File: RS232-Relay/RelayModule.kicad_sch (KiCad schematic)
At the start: 30 parts, among them J9 Relay 1-4, K1 G5V-1, K2 G5V-1, K3 G5V-1, K4 G5V-1, Q1 2N3904, Q2 2N3904, Q3 2N3904, Q4 2N3904, U6 LTV-847S

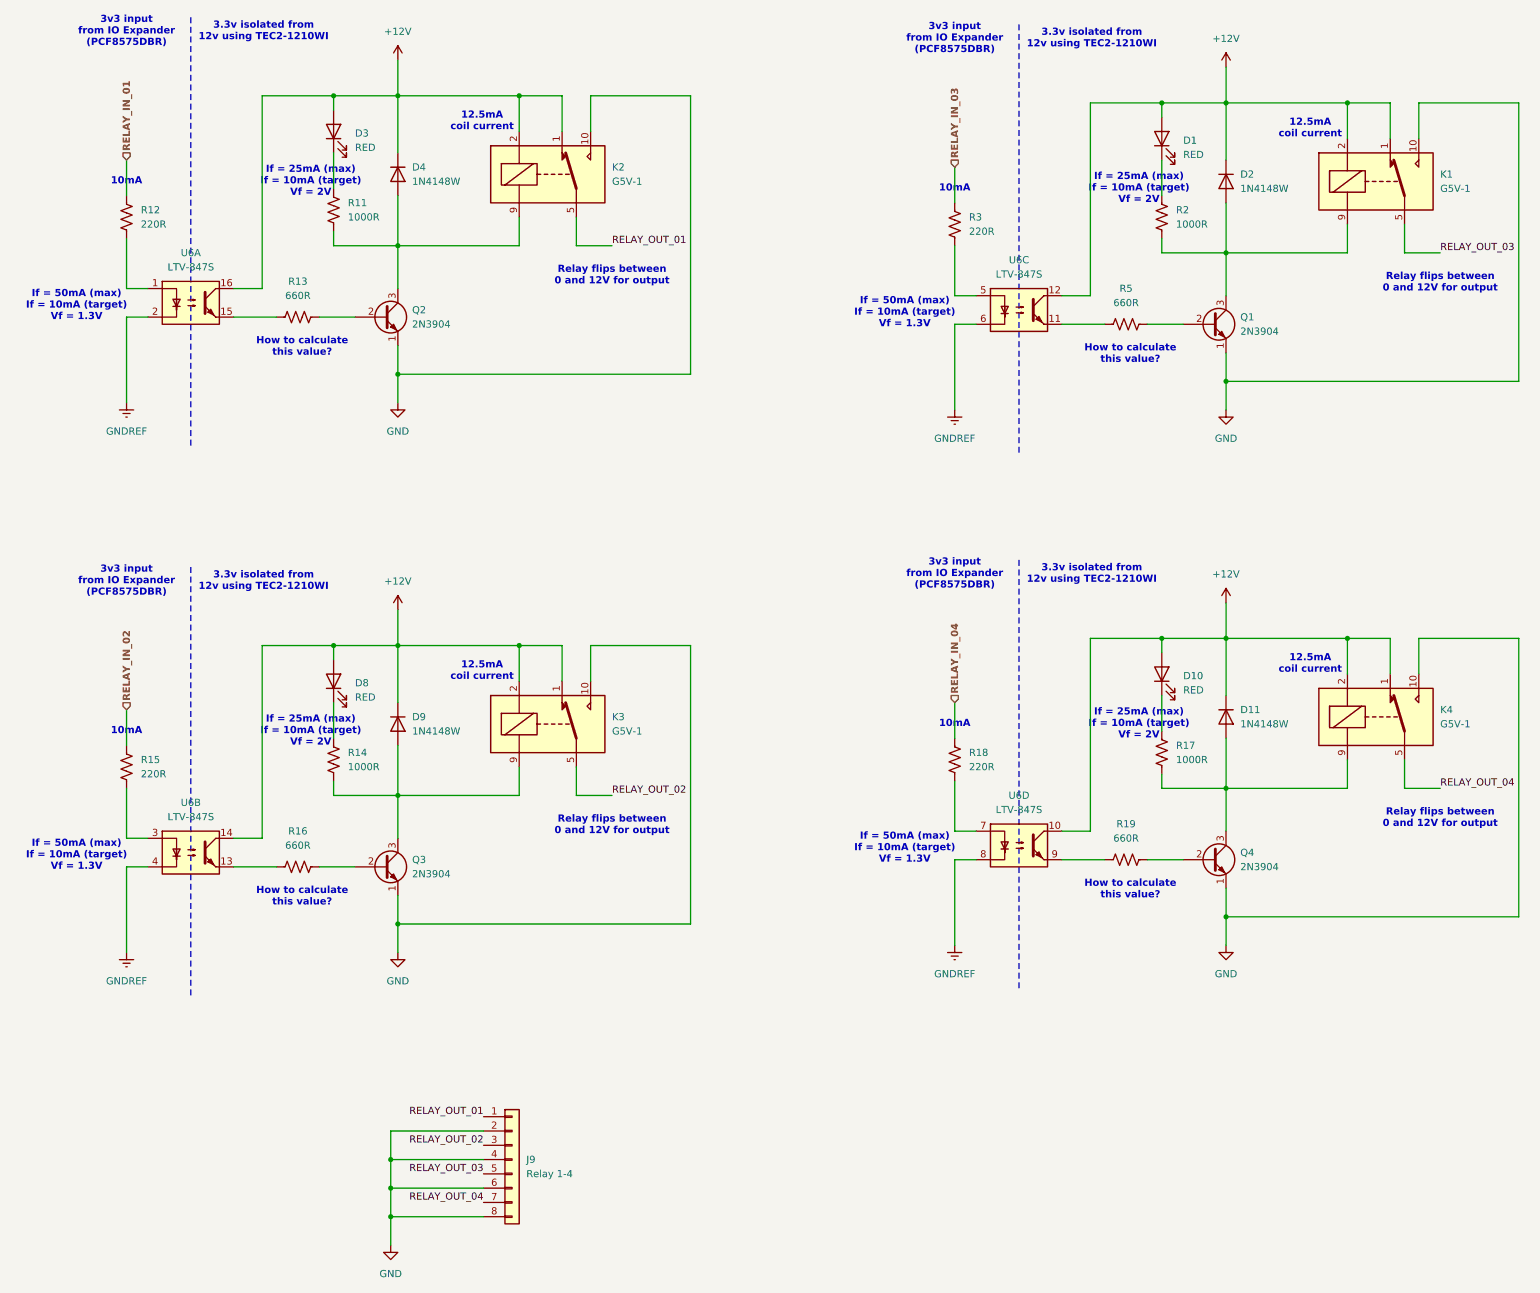
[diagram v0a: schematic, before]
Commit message: 1x Layout Complete
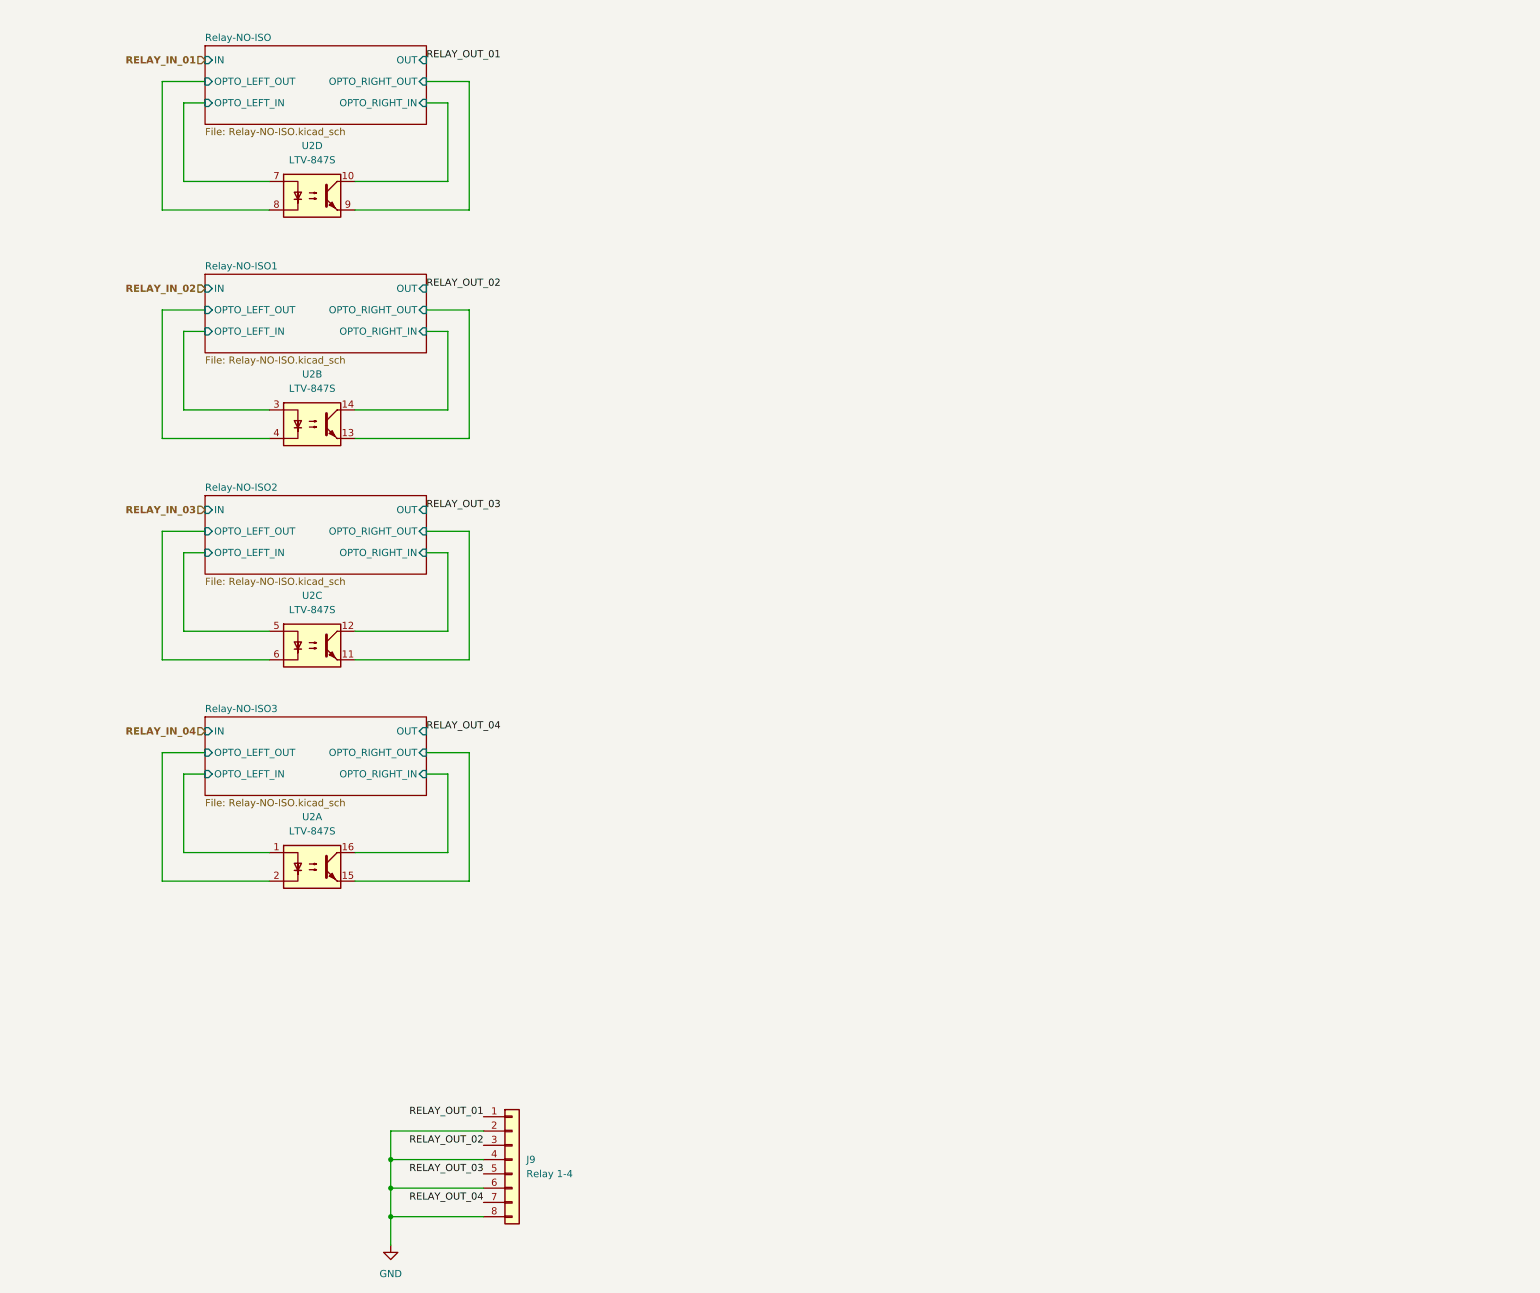
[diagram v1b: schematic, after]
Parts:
- removed D1, D10, D3, D8: RED, LED_SMD:LED_0805_2012Metric, symbol Device:LED
- removed D11, D2, D4, D9: 1N4148W, Diode_SMD:D_SOD-123, symbol Device:D
- removed K1, K2, K3, K4: G5V-1, Relay_THT:Relay_SPDT_Omron_G5V-1, symbol Relay:G5V-1
- removed Q1, Q2, Q3, Q4: 2N3904, Package_TO_SOT_SMD:SOT-23, symbol Transistor_BJT:2N3904
- removed R11, R14, R17, R2: 1000R, Resistor_SMD:R_0603_1608Metric, symbol Device:R_US
- removed R12, R15, R18, R3: 220R, Resistor_SMD:R_0603_1608Metric, symbol Device:R_US
- removed R13, R16, R19, R5: 660R, Resistor_SMD:R_0603_1608Metric, symbol Device:R_US
- removed U6: LTV-847S, Package_DIP:SMDIP-16_W9.53mm, symbol Isolator:LTV-847S
- added U2: LTV-847S, Package_DIP:SMDIP-16_W9.53mm, symbol Isolator:LTV-847S
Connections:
- new net Relay-NO-ISO/OPTO_LEFT_IN: U2.7
- new net Relay-NO-ISO/OPTO_LEFT_OUT: U2.8
- new net Relay-NO-ISO/OPTO_RIGHT_IN: U2.10
- new net Relay-NO-ISO/OPTO_RIGHT_OUT: U2.9
- new net Relay-NO-ISO1/OPTO_LEFT_IN: U2.3
- new net Relay-NO-ISO1/OPTO_LEFT_OUT: U2.4
- new net Relay-NO-ISO1/OPTO_RIGHT_IN: U2.14
- new net Relay-NO-ISO1/OPTO_RIGHT_OUT: U2.13
- new net Relay-NO-ISO2/OPTO_LEFT_IN: U2.5
- new net Relay-NO-ISO2/OPTO_LEFT_OUT: U2.6
- new net Relay-NO-ISO2/OPTO_RIGHT_IN: U2.12
- new net Relay-NO-ISO2/OPTO_RIGHT_OUT: U2.11
- new net Relay-NO-ISO3/OPTO_LEFT_IN: U2.1
- new net Relay-NO-ISO3/OPTO_LEFT_OUT: U2.2
- new net Relay-NO-ISO3/OPTO_RIGHT_IN: U2.16
- new net Relay-NO-ISO3/OPTO_RIGHT_OUT: U2.15
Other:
- added sheet Relay-NO-ISO (Relay-NO-ISO.kicad_sch)
- added sheet Relay-NO-ISO1 (Relay-NO-ISO.kicad_sch)
- added sheet Relay-NO-ISO2 (Relay-NO-ISO.kicad_sch)
- added sheet Relay-NO-ISO3 (Relay-NO-ISO.kicad_sch)
- note removed: "10mA"
- note removed: "12.5mA coil current"
- note removed: "3.3v isolated from 12v using TEC2-1210WI"
- note removed: "3v3 input from IO Expander (PCF8575DBR)"
- note removed: "How to calculate this value?"
- note removed: "If = 25mA (max) If = 10mA (target) Vf = 2V"
- note removed: "If = 50mA (max) If = 10mA (target) Vf = 1.3V"
- note removed: "Relay flips between 0 and 12V for output"
